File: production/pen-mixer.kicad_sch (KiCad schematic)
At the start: 28 parts, among them J1 USB-C 16P, J2 BAT, U1 ISP1807-LR, U2 LSM6DS3TR-C, U3 MCP73831T-2ACI/OT, U4 TPS7A0533PDBV

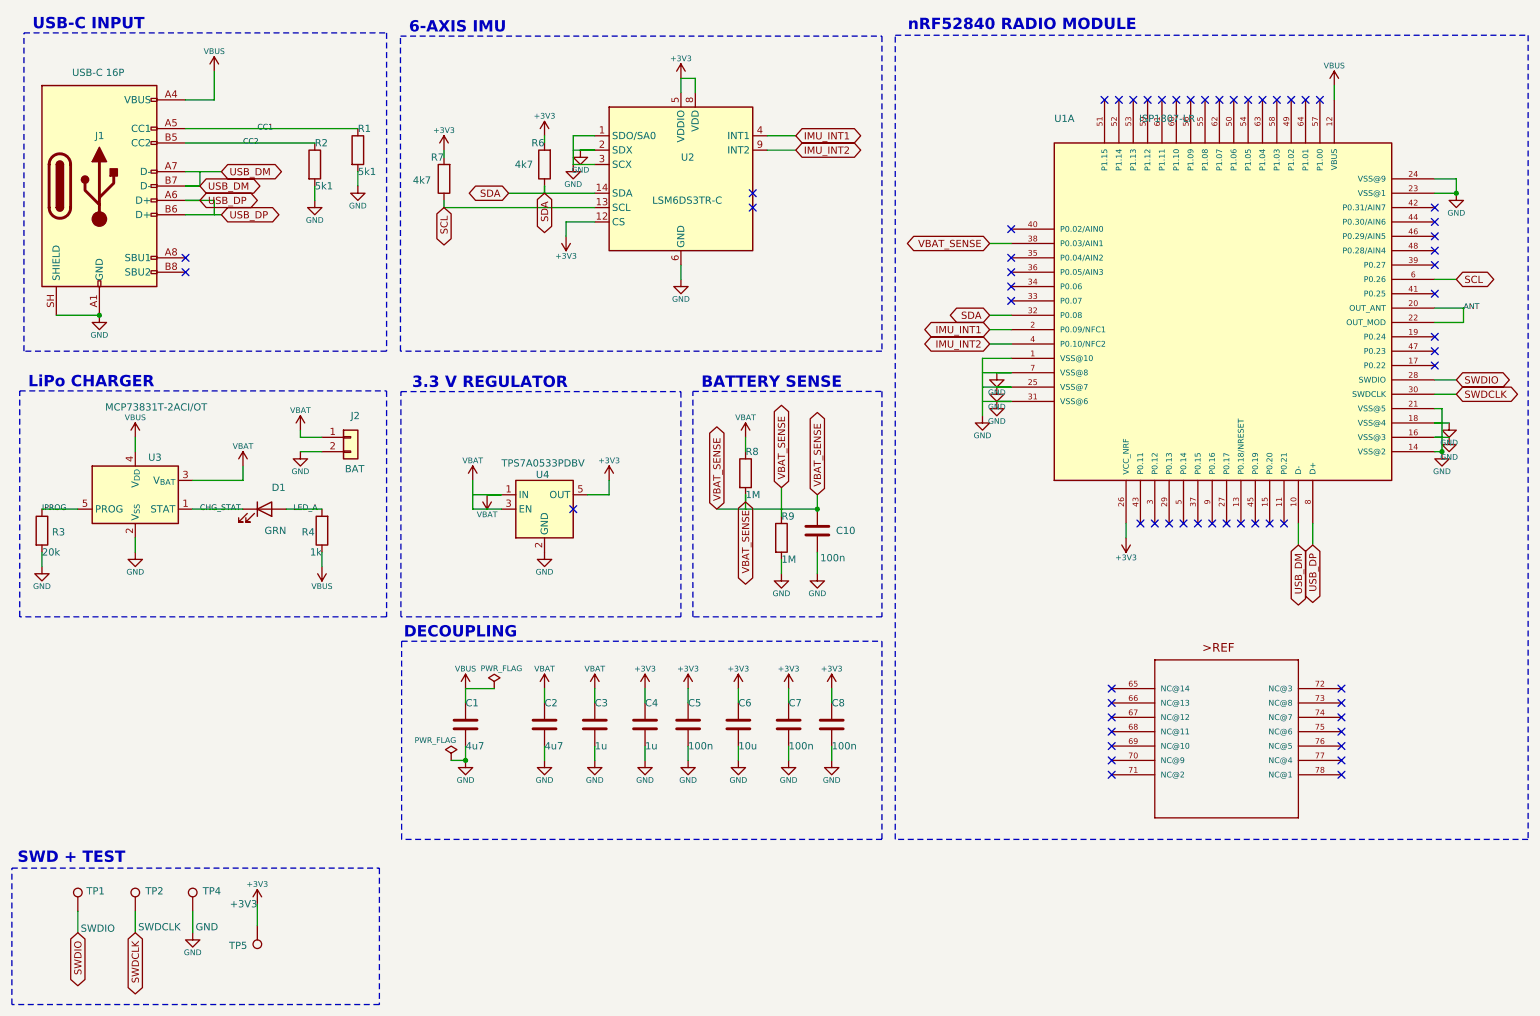
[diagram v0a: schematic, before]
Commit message: pads to board extremes
Claude-Session: https://claude.ai/code/session_01RCYT2QSY7BVZDeTyE9KrC4
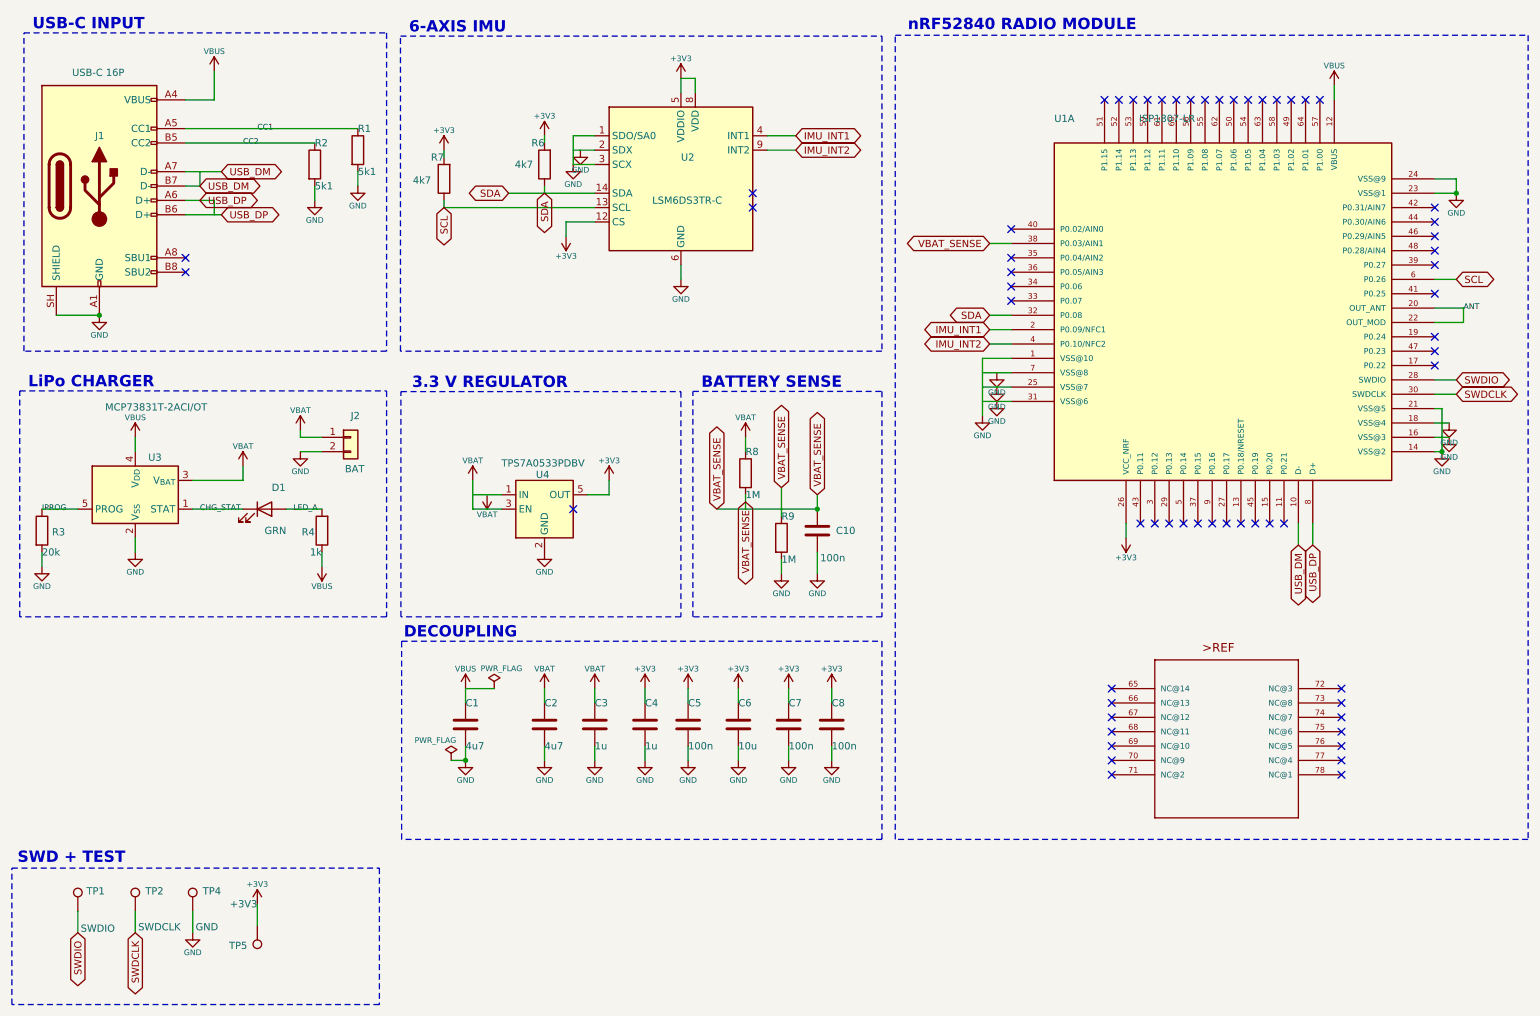
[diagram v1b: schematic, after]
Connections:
- net GND: no longer U1.25 (VSS@7), U1.31 (VSS@6), U1.7 (VSS@8), U2.2 (SDX)
- net VBAT: no longer U4.1 (IN)
